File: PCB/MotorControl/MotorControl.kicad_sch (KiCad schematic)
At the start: 11 parts, among them J1 Conn_01x05_Pin, J5 Conn_01x05_Pin, J6 USB_C_Receptacle_USB2.0_14P, J8 Conn_01x04_Socket, U1 PCA9685PW, U3 TC1262-33, U4 STM32L031K6Tx

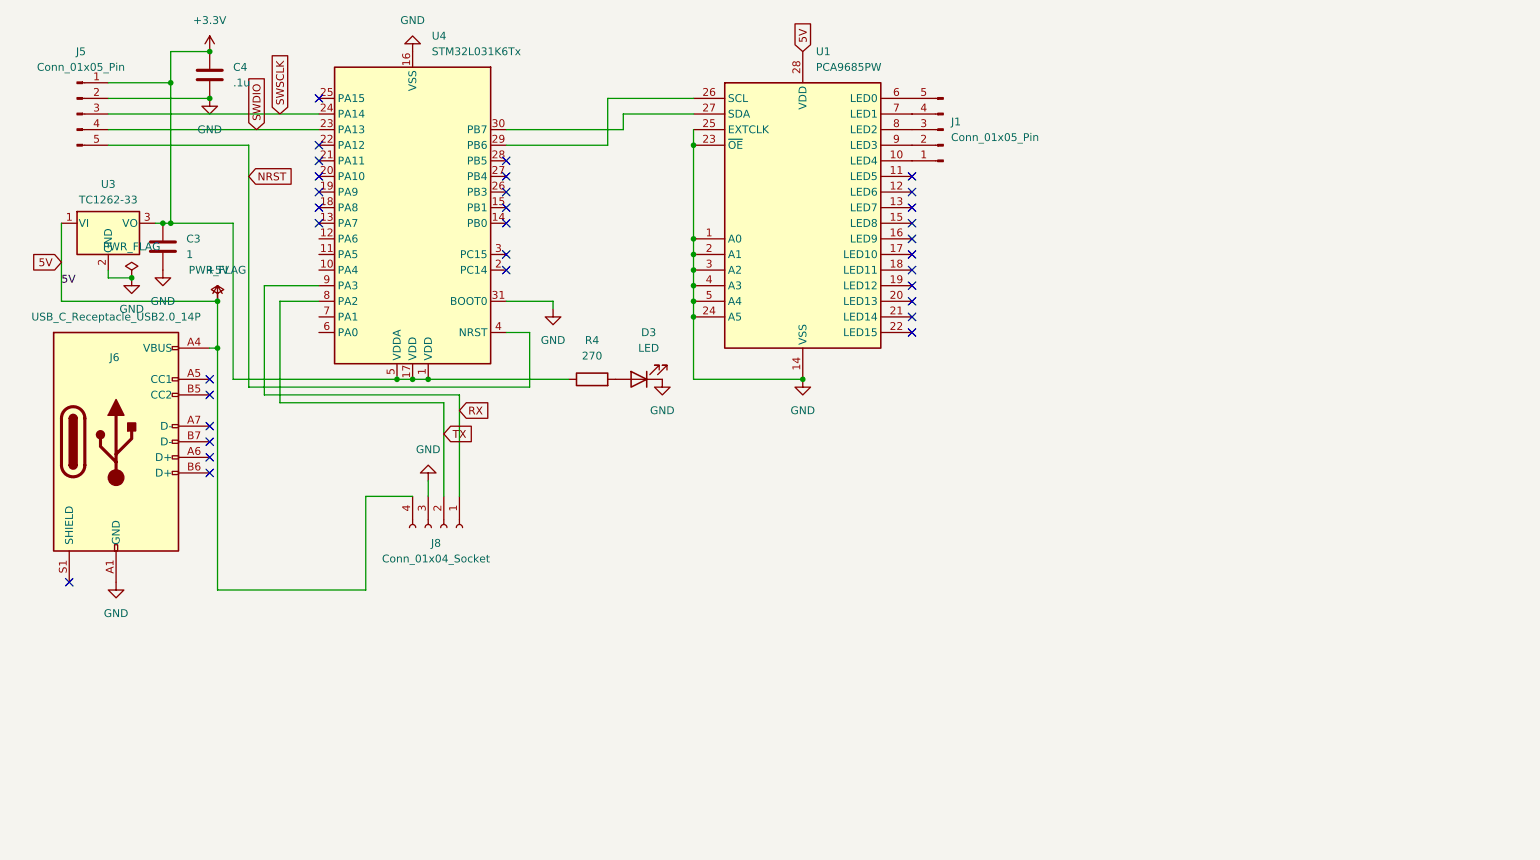
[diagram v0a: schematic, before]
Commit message: Pushing
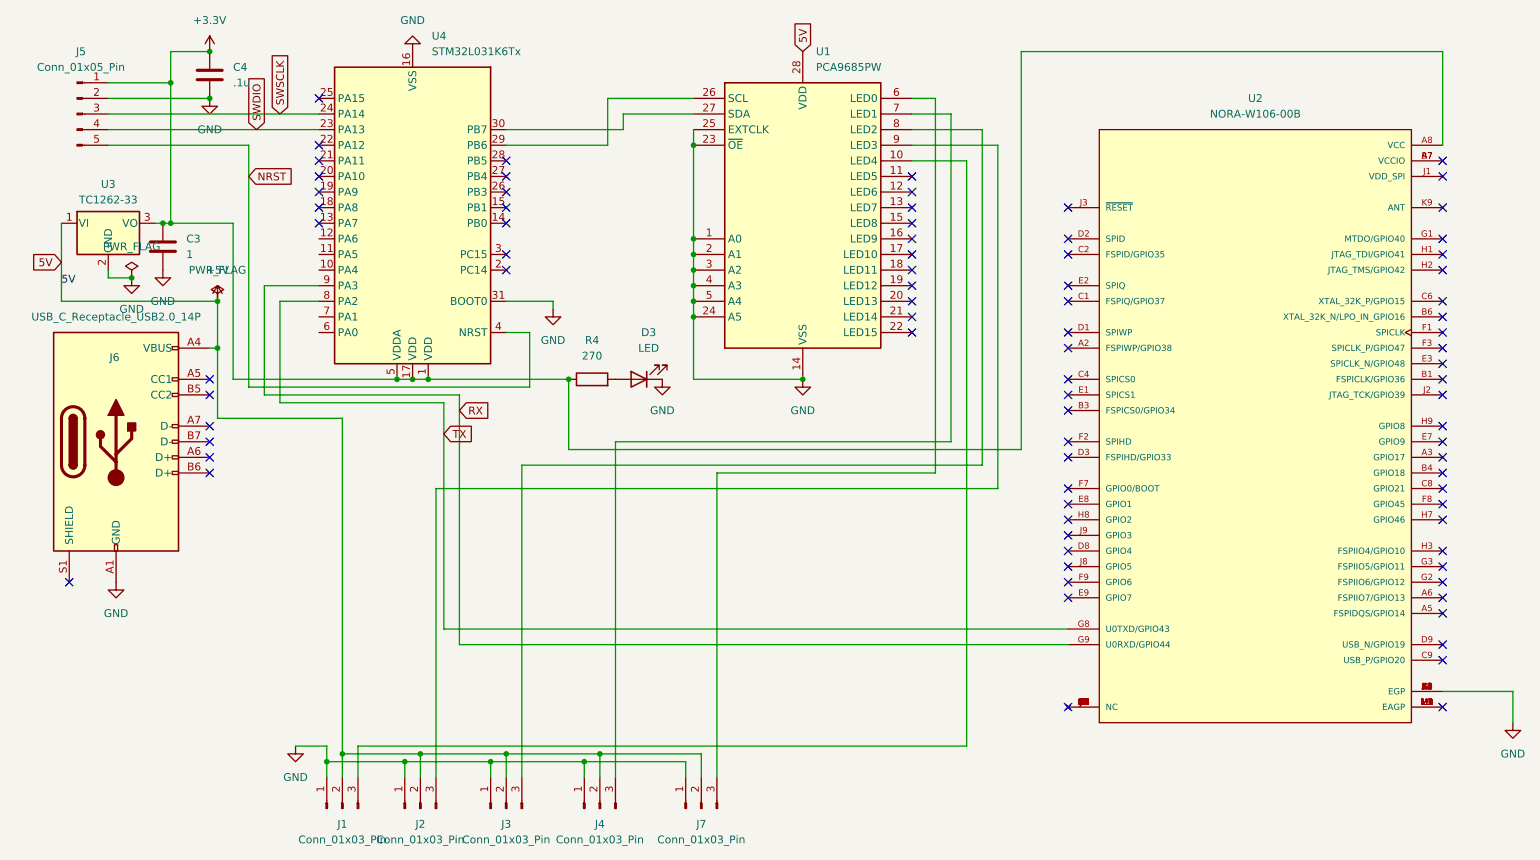
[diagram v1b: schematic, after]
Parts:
- removed J1: Conn_01x05_Pin, Connector_PinHeader_1.00mm:PinHeader_1x05_P1.00mm_Vertical, symbol Connector:Conn_01x05_Pin
- removed J8: Conn_01x04_Socket, Connector_PinHeader_1.00mm:PinHeader_1x04_P1.00mm_Horizontal, symbol Connector:Conn_01x04_Socket
- added J1, J2, J3, J4, J7: Conn_01x03_Pin, Connector_PinHeader_2.54mm:PinHeader_1x03_P2.54mm_Horizontal, symbol Connector:Conn_01x03_Pin
- added U2: NORA-W106-00B, NORA-W106-00B:XCVR_NORA-W106-00B, symbol NORA-W106-00B:NORA-W106-00B
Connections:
- net +3.3V: now also U2.A8 (VCC)
- net +5V: now also J1.2 (Pin_2), J2.2 (Pin_2), J3.2 (Pin_2), J4.2 (Pin_2), J7.2 (Pin_2)
- net GND: now also J1.1 (Pin_1), J2.1 (Pin_1), J3.1 (Pin_1), J4.1 (Pin_1), J7.1 (Pin_1), U2.A1 (EGP), U2.A9 (EGP), U2.B2 (EGP), U2.B8 (EGP), U2.E4 (EGP), U2.E5 (EGP), U2.F4 (EGP), U2.F5 (EGP), U2.K2 (EGP), U2.K3 (EGP), U2.K5 (EGP), U2.K7 (EGP), U2.K8 (EGP)
- net RX: now also U2.G9 (U0RXD/GPIO44)
- net TX: now also U2.G8 (U0TXD/GPIO43)
- net at U1.10 (LED4): now also J1.3 (Pin_3)
- net at U1.9 (LED3): now also J2.3 (Pin_3)
- net at U1.8 (LED2): now also J3.3 (Pin_3)
- net at U1.7 (LED1): now also J4.3 (Pin_3)
- net at U1.6 (LED0): now also J7.3 (Pin_3)
- new net: U2.A4 (NC), U2.B5 (NC), U2.B9 (NC), U2.C5 (NC), U2.D7 (NC), U2.G4 (NC), U2.G5 (NC), U2.G7 (NC), U2.J4 (NC), U2.J5 (NC), U2.J7 (NC), U2.K1 (NC)
- new net: U2.A7 (VCCIO), U2.B7 (VCCIO)
- new net: U2.L1 (EAGP), U2.L9 (EAGP), U2.M1 (EAGP), U2.M2 (EAGP), U2.M8 (EAGP), U2.M9 (EAGP)
- no-connect marks 32 -> 81
